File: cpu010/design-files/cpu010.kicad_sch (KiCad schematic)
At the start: 8 parts, among them U101 GAL22V10

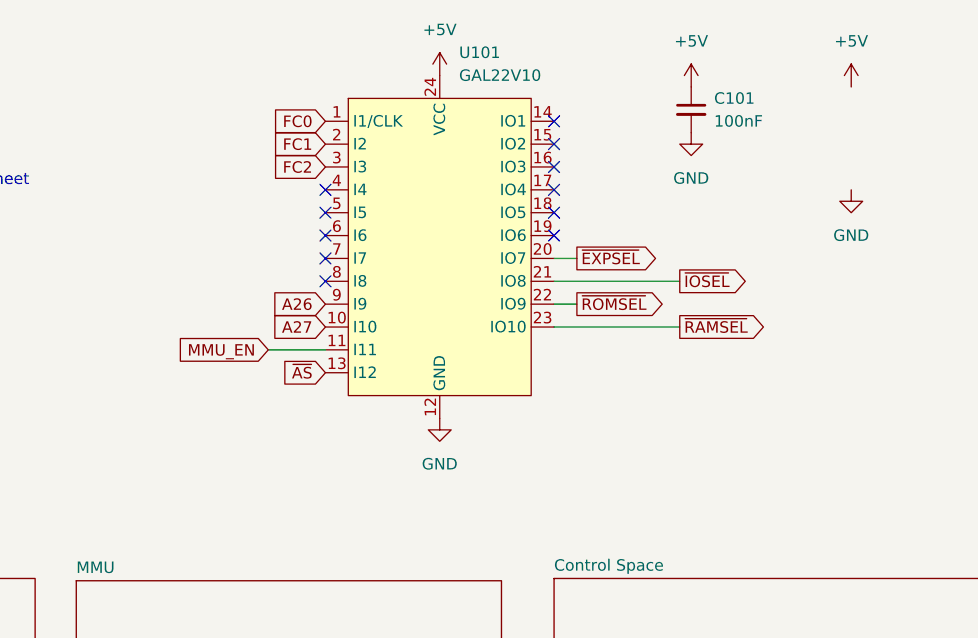
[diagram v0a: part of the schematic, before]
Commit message: Routing some I/O stuff.
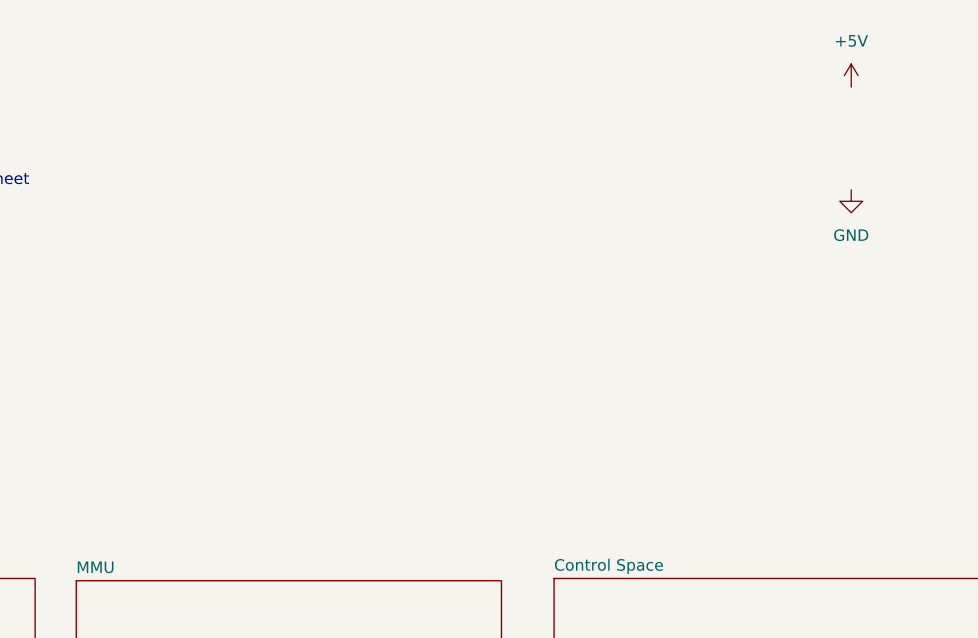
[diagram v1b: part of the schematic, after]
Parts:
- removed C101: 100nF, Capacitor_SMD:C_0805_2012Metric_Pad1.18x1.45mm_HandSolder, symbol Device:C_Small
- removed U101: GAL22V10, Package_DIP:DIP-24_W7.62mm_Socket, symbol jrt-ICs:GAL22V10
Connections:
- no-connect marks 11 -> 0
